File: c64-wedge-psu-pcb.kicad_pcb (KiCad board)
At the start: 2 copper layers, 70 x 54 mm, 22 parts, among them U1 LM2576T-ADJ

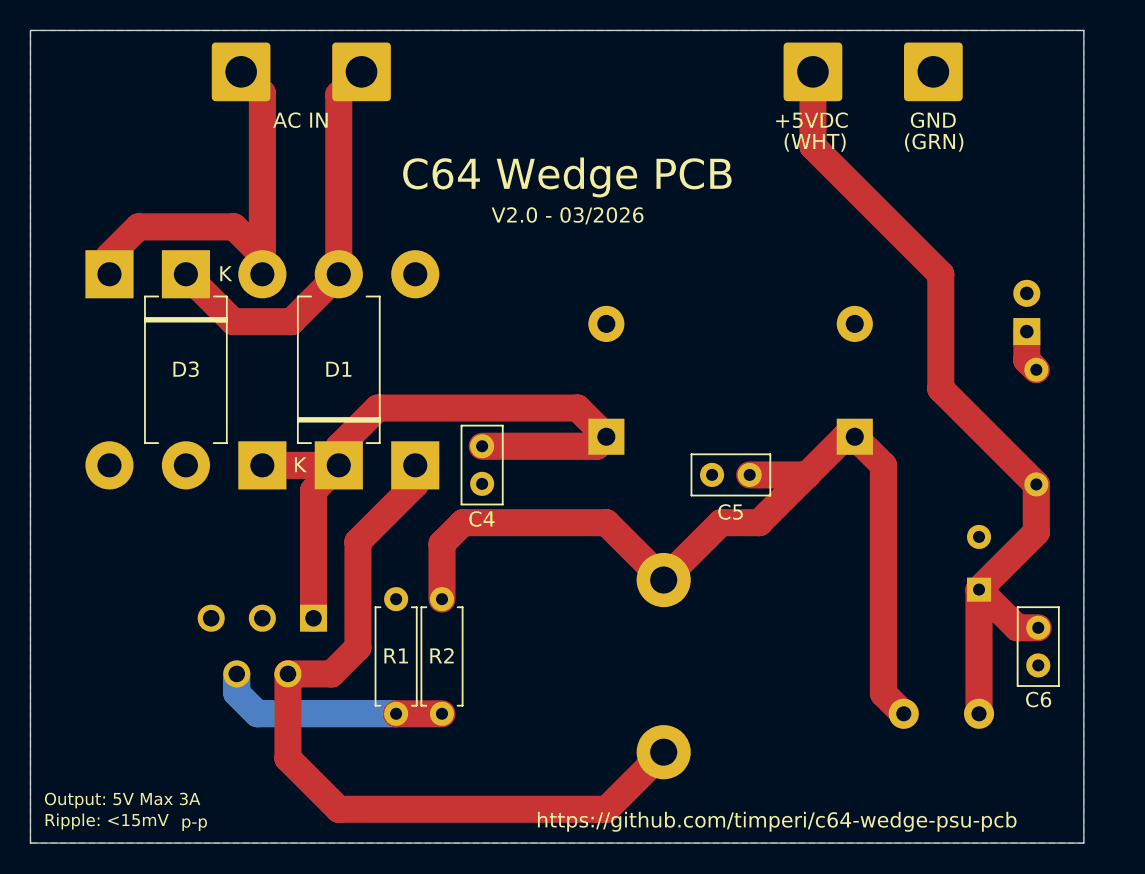
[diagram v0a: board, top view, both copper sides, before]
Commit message: updates
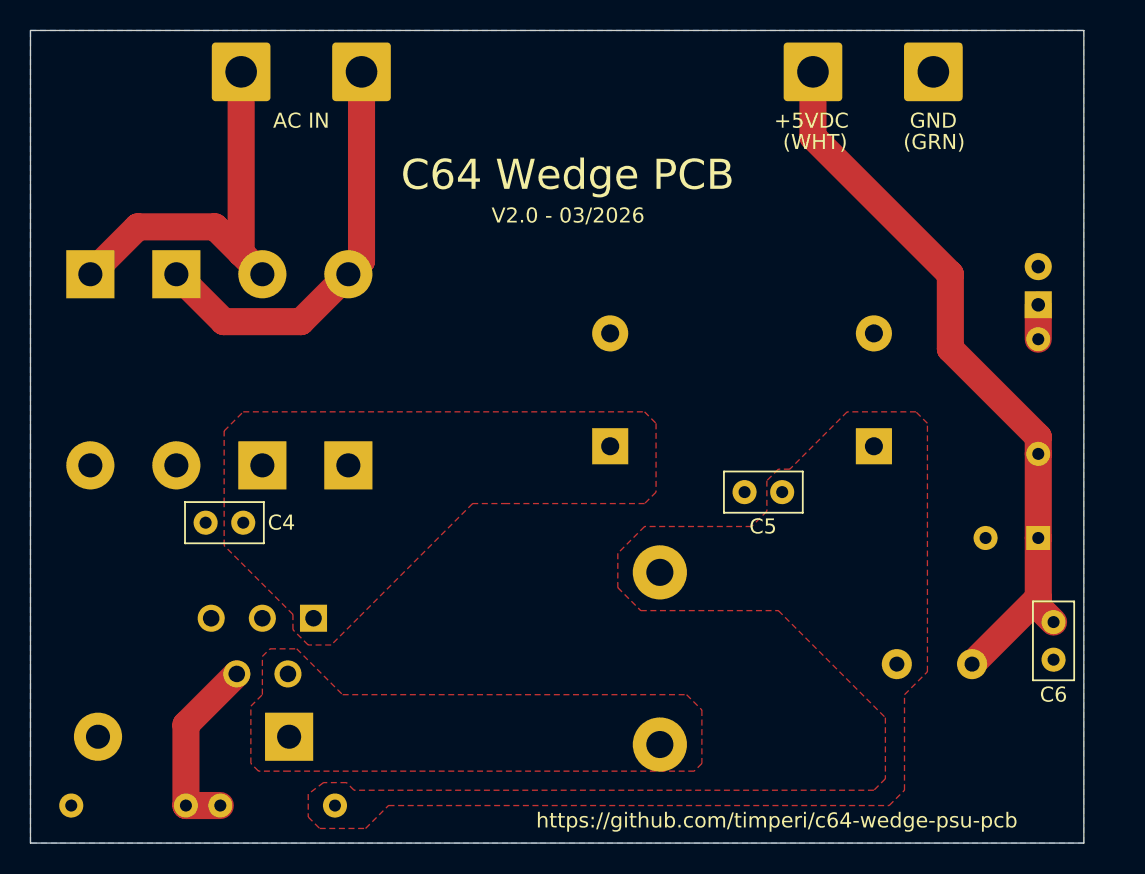
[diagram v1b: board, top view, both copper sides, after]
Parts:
- C1: footprint Capacitor_THT:CP_Radial_D16.0mm_P7.50mm -> Capacitor_THT:CP_Radial_D18.0mm_P7.50mm
- D1, D3, R1, R2: moved to B.Cu
- moved D5 19.9 mm to (107.2, 106.9), turned to 180 degrees
- moved C4 16.7 mm to (104.1, 92.7), turned to 180 degrees
- moved R2 15.5 mm to (110.2, 111.5), turned to 180 degrees
- moved R1 15.2 mm to (100.3, 111.5), turned to 180 degrees
- moved C3 5.22 mm to (157.0, 93.7), turned to 180 degrees
- moved L2 3.33 mm to (150.1, 102.1)
- moved C5 2.44 mm to (140.0, 90.7)
- moved R3 2.04 mm to (157.0, 88.1)
- moved LED1 1.93 mm to (157.0, 78.2)
- moved C2 1.42 mm to (146.1, 87.6)
- moved D4 1.27 mm to (94.0, 76.2)
- moved C6 1.09 mm to (158.0, 99.3)
- moved C1 0.68 mm to (128.5, 87.6)
- moved D1 0.64 mm to (111.1, 88.9)
- moved D3 0.64 mm to (99.7, 76.2)
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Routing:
- net Net-(C2-Pad1): track 60.8 -> 0.00 mm
- net Net-(D5-K): track 52.6 -> 0.11 mm
- net Net-(D1-K): track 45.3 -> 0.00 mm
- net /+5VDC: track 55.4 -> 49.4 mm
- net Net-(U1-FB): track 15.5 -> 12.4 mm
- net Net-(D2-A): track 28.9 -> 26.7 mm
- net Net-(D1-A): track 26.8 -> 27.9 mm
- net Net-(LED1-Pin_1): track 2.80 -> 2.29 mm
- added copper zone on F.Cu, net Net-(C2-Pad1)
- added copper zone on F.Cu, net Net-(D1-K)
- added copper zone on F.Cu, net Net-(D5-K)
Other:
- board text removed: "Output: 5V Max 3A"
- board text removed: "Ripple: <15mV"
- board text removed: "p-p"
